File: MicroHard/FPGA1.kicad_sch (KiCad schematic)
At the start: 2 parts, among them IC1 S25FL512SAGMFI011, U4 XC7A100T-FTG256

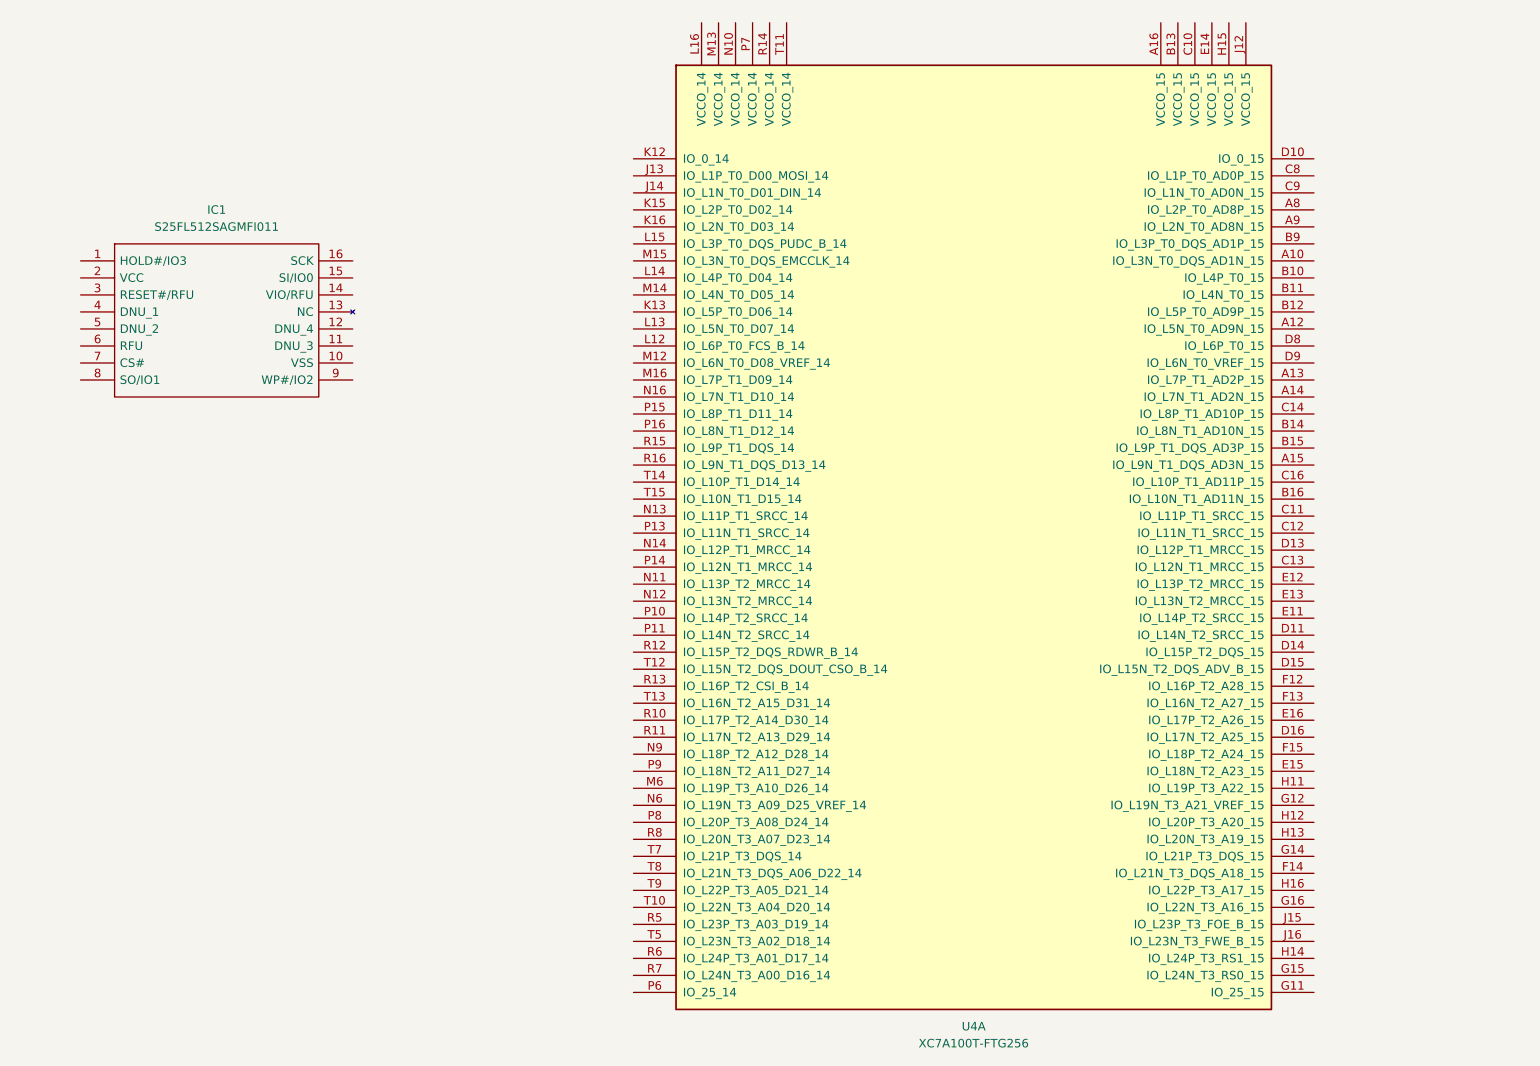
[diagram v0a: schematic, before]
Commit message: feat: finished Flash mem and FPGA Config
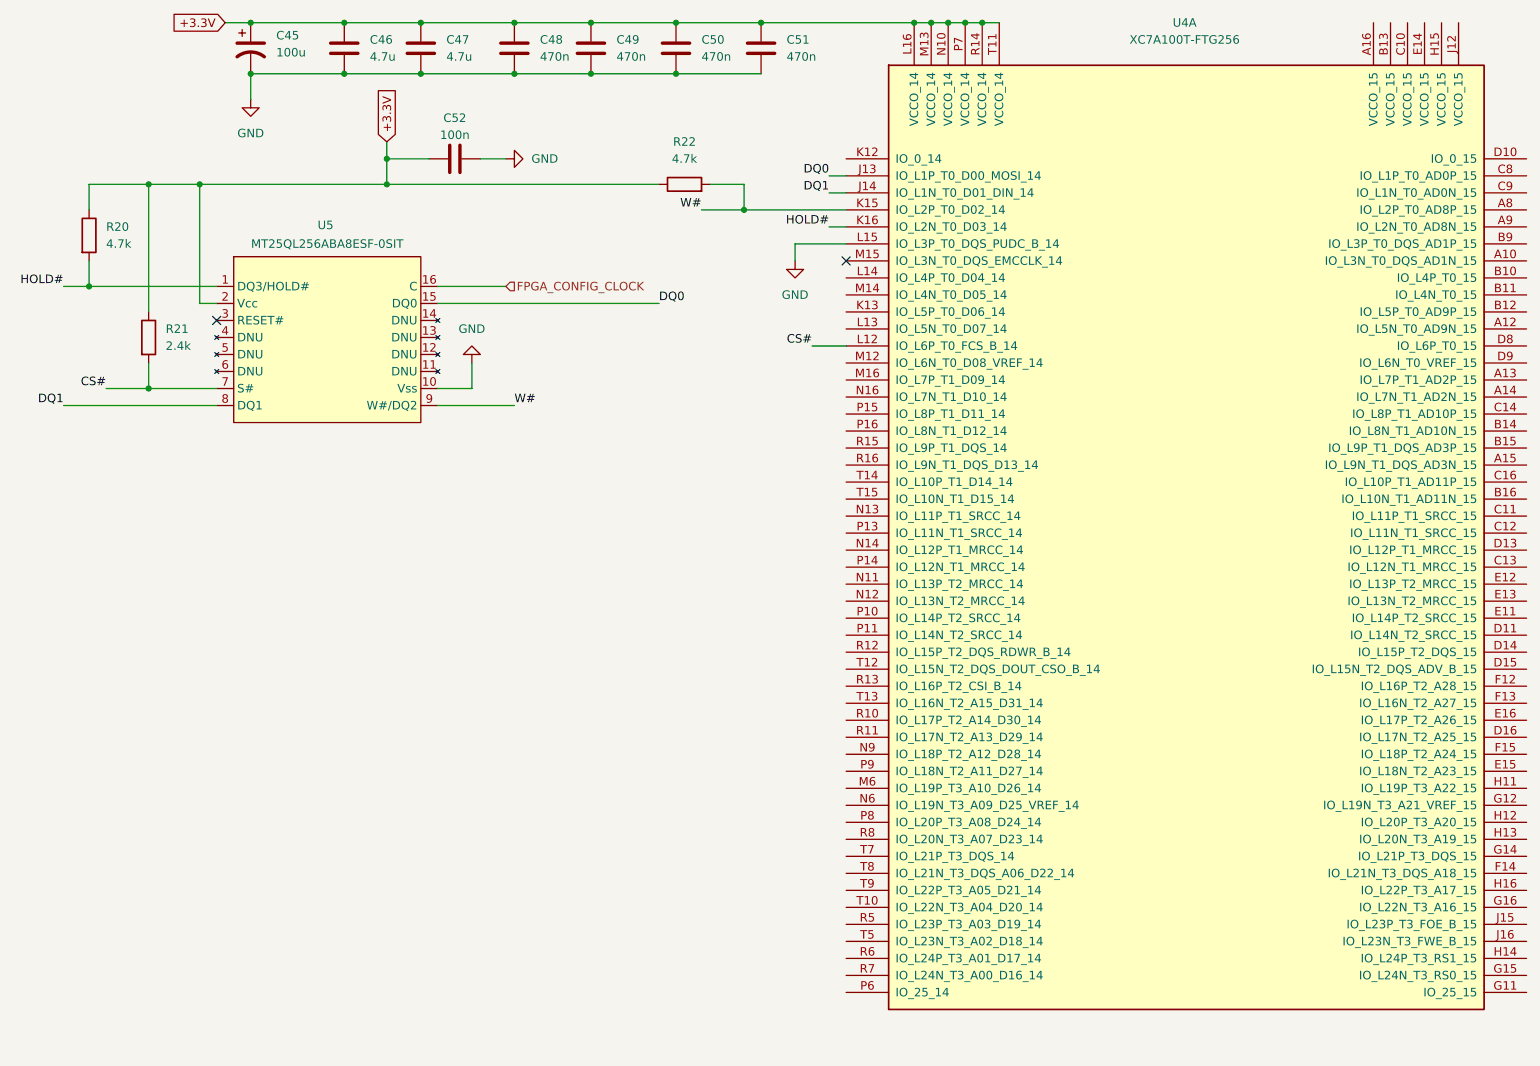
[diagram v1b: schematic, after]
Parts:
- removed IC1: S25FL512SAGMFI011, SOIC127P1030X265-16N, symbol S25FL512SAGMFI011:S25FL512SAGMFI011
- added C45: 100u, symbol Device:C_Polarized_US
- added C46, C47: 4.7u, symbol Device:C
- added C48, C49, C50, C51: 470n, symbol Device:C
- added C52: 100n, symbol Device:C
- added R20, R22: 4.7k, symbol Device:R
- added R21: 2.4k, symbol Device:R
- added U5: MT25QL256ABA8ESF-0SIT, symbol MicroHardLibrary:MT25QL256ABA8ESF-0SIT
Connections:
- net DQ0: now reaches U4.J13 (IO_L1P_T0_D00_MOSI_14)
- net DQ0: now also U5.15 (DQ0)
- net DQ1: now reaches U4.J14 (IO_L1N_T0_D01_DIN_14)
- net DQ1: now also U5.8 (DQ1)
- net W#: now reaches U4.K15 (IO_L2P_T0_D02_14)
- net W#: now also R22.2, U5.9 (W#/DQ2)
- net HOLD#: now reaches U4.K16 (IO_L2N_T0_D03_14)
- net HOLD#: now also R20.2, U5.1 (DQ3/HOLD#)
- net CS#: now reaches U4.L12 (IO_L6P_T0_FCS_B_14)
- net CS#: now also R21.2, U5.7 (S#)
- net GND: now reaches U4.L15 (IO_L3P_T0_DQS_PUDC_B_14)
- net GND: now also C45.2, C46.2, C47.2, C48.2, C49.2, C50.2, C51.2, C52.2, U5.10 (Vss)
- net +3.3V: now reaches U4.L16 (VCCO_14)
- net +3.3V: now also U4.M13 (VCCO_14), U4.N10 (VCCO_14), U4.P7 (VCCO_14), U4.R14 (VCCO_14), U4.T11 (VCCO_14), C45.1, C46.1, C47.1, C48.1, C49.1, C50.1, C51.1, C52.1, R20.1, R21.1, R22.1, U5.2 (Vcc)
- new net FPGA_CONFIG_CLOCK: U5.16 (C)
- no-connect marks 0 -> 2
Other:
- moved on the sheet: U4A
